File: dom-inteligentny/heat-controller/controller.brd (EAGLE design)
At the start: 92.2 x 87.3 mm, 43 parts, among them IC1 24C64SM, IC2 DS3231/SO, K1 691218410002, K2 691218410002, K3 691218410002, T1 BC847, T10 BC847, T11 BC847, T12 BC847, T2 BC847, T3 BC847, T4 BC847, T5 BC847, T6 BC847, T7 BC847, T8 BC847, T9 BC847, U1 MAX3485ECSA+T, X1 TERMINAL-BLOCK-3.5MM-6-PIN-LO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, X2 TERMINAL-BLOCK-3.5MM-6-PIN-LO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, X3 TERMINAL-BLOCK-3.5MM-3-PIN-LO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, X4 JST-XH-05-PIN-LONG-PAD, X5 GLX-S-88M

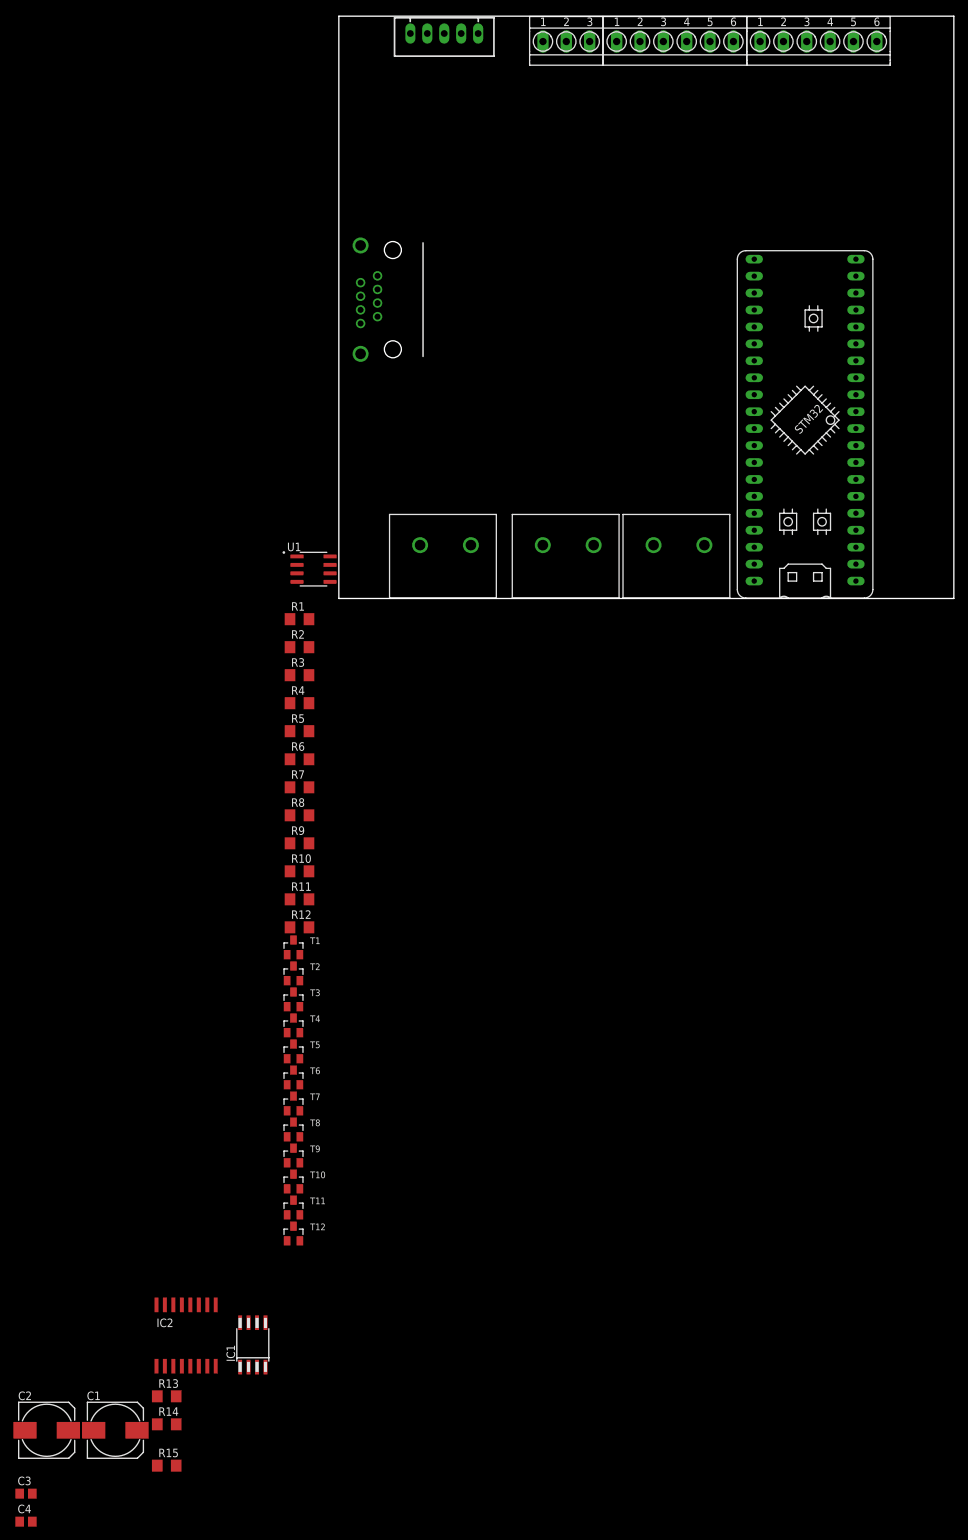
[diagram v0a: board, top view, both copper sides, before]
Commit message: MLU board
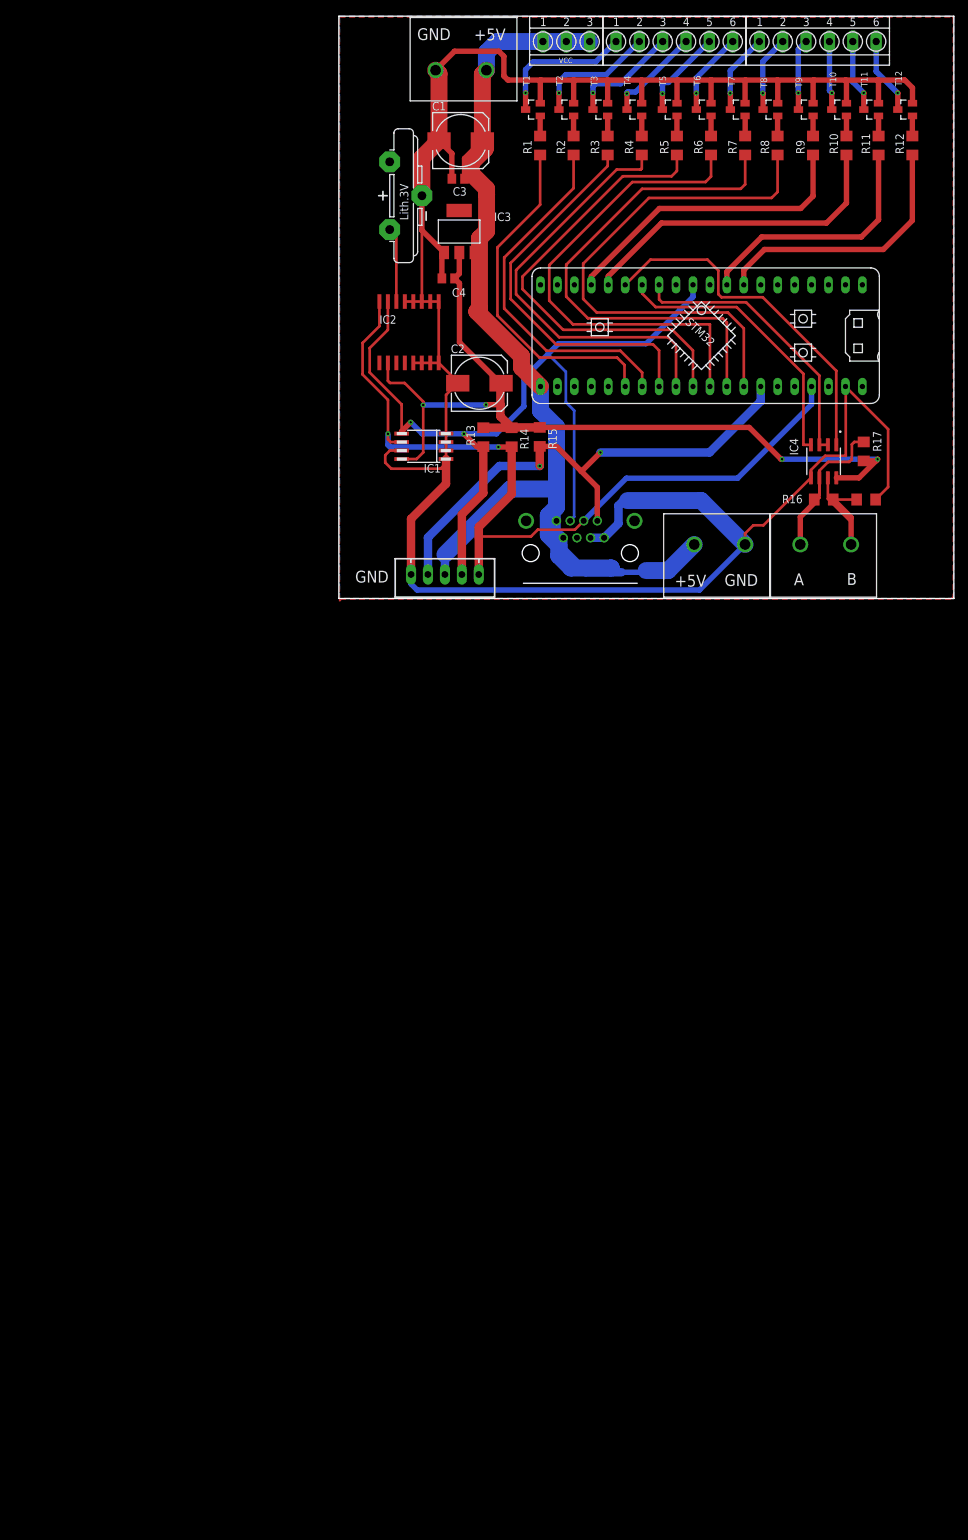
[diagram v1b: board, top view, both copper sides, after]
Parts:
- removed U1: MAX3485ECSA+T, MAX3485ECSA_T:SOIC127P600X175-8N
- added G1: CR2032V, battery:CR2032V
- added IC3: REG1117, burr-brown:SOT223
- added IC4: MAX3485ECSA+T, MAX3485ECSA_T:SOIC127P600X175-8N
- added R16: R120, eagle-ltspice:R1206
- added R17, R18: 20K, eagle-ltspice:R1206
- IC1: value 24C64SM -> FM24CL64B
- IC2: value DS3231/SO -> DS3231
- moved C3 207.5 mm to (17.9, 62.9), turned to 180 degrees
- moved C1 200.2 mm to (18.3, 68.6)
- moved C4 196.8 mm to (16.4, 48.0)
- moved T12 191.8 mm to (84.9, 73.3), turned to 90 degrees
- moved T11 186.0 mm to (79.8, 73.3), turned to 90 degrees
- moved T10 180.3 mm to (75.0, 73.3), turned to 90 degrees
- moved T9 174.6 mm to (70.0, 73.3), turned to 90 degrees
- moved C2 169.8 mm to (21.1, 32.3)
- moved T8 168.8 mm to (64.7, 73.3), turned to 90 degrees
- moved R15 164.1 mm to (30.1, 24.2), turned to 270 degrees
- moved T7 163.2 mm to (59.8, 73.3), turned to 90 degrees
- moved T6 157.6 mm to (54.7, 73.3), turned to 90 degrees
- moved R14 156.7 mm to (25.9, 24.2), turned to 270 degrees
- moved IC2 154.1 mm to (10.5, 39.9)
- moved T5 152.0 mm to (49.6, 73.3), turned to 90 degrees
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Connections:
- removed net N$1: K3.1, U1.6
- removed net N$2: K3.2, U1.7
- removed net VBAT: IC2.14
- new net A: IC4.6, K3.1, R16.1, R17.1
- new net B: IC4.7, K3.2, R16.2, R18.2
- new net N$3: G1.+, IC2.14
- net 3V: now also IC3.2, IC4.8, R17.2; no longer U$1.P$20, U1.8
- net GND: now also G1.-, IC3.1, IC4.5, R18.1; no longer U1.5
- net N$15: now also U$1.P$17; no longer U$1.P$16
- net N$16: now also U$1.P$16; no longer U$1.P$17
- net N$17: now also U$1.P$9; no longer U$1.P$8
- net N$18: now also U$1.P$8; no longer U$1.P$9
- net N$4: now also IC4.2, IC4.3; no longer U1.2, U1.3
- net N$5: now also IC4.4; no longer U1.4
- net N$6: now also IC4.1; no longer U1.1
- net VCC: now also IC3.3
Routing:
- net GND: track 0.00 -> 379.5 mm
- net VCC: track 0.00 -> 189.0 mm
- net 3V: track 0.00 -> 133.0 mm, vias 0 -> 4
- net SDA: track 0.00 -> 131.8 mm, vias 0 -> 2
- net SCL: track 0.00 -> 127.9 mm, vias 0 -> 2
- net INT: track 0.00 -> 79.4 mm, vias 0 -> 2
- net N$14: track 0.00 -> 79.0 mm
- net N$13: track 0.00 -> 76.3 mm
- net N$12: track 0.00 -> 73.2 mm
- net N$11: track 0.00 -> 68.8 mm
- net N$10: track 0.00 -> 64.1 mm
- net N$9: track 0.00 -> 58.5 mm
- net N$8: track 0.00 -> 54.1 mm
- net N$6: track 0.00 -> 53.3 mm
- net N$7: track 0.00 -> 52.1 mm
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- added copper zone on layer 1, net GND
- added copper zone on layer 16, net GND
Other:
- board text added: "+5V"
- board text added: "A"
- board text added: "B"
- board text added: "GND"
- board text added: "MAIN LOGIC UNIT v 1.0 falcon IoT https://falcon.software https://weblogic.pl"
- board text added: "VCC"
